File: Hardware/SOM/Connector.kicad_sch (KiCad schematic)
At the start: 1 part, among them J1 SODIMM-200_Split

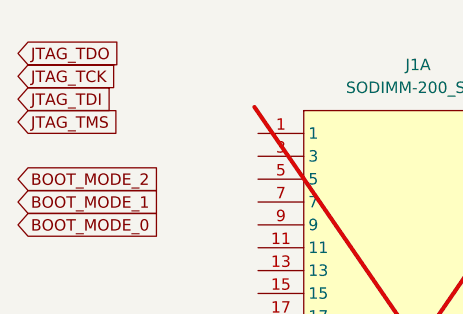
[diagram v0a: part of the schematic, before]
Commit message: DDR Banks Vref
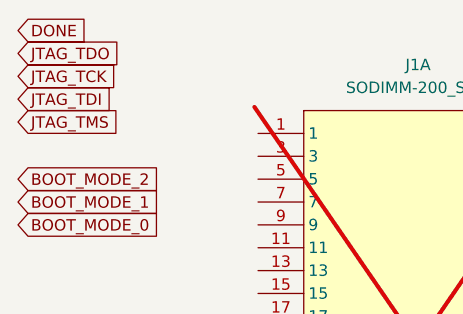
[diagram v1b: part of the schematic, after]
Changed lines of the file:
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@@
+		)
+	)
+	(global_label "DONE"
+		(shape input)
+		(at 19.05 19.05 0)
+		(fields_autoplaced yes)
+		(effects
+			(font
+				(size 1.27 1.27)
+			)
+			(justify left)
+		)
+		(property "Intersheetrefs" "${INTERSHEET_REFS}"
+			(at 27.1152 19.05 0)
+			(effects
+				(font
+					(size 1.27 1.27)
+				)
+				(justify left)
+				(hide yes)
+			)
 		)
 	)
